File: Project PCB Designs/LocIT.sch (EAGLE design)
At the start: 5 parts, among them J1 PRT-14017

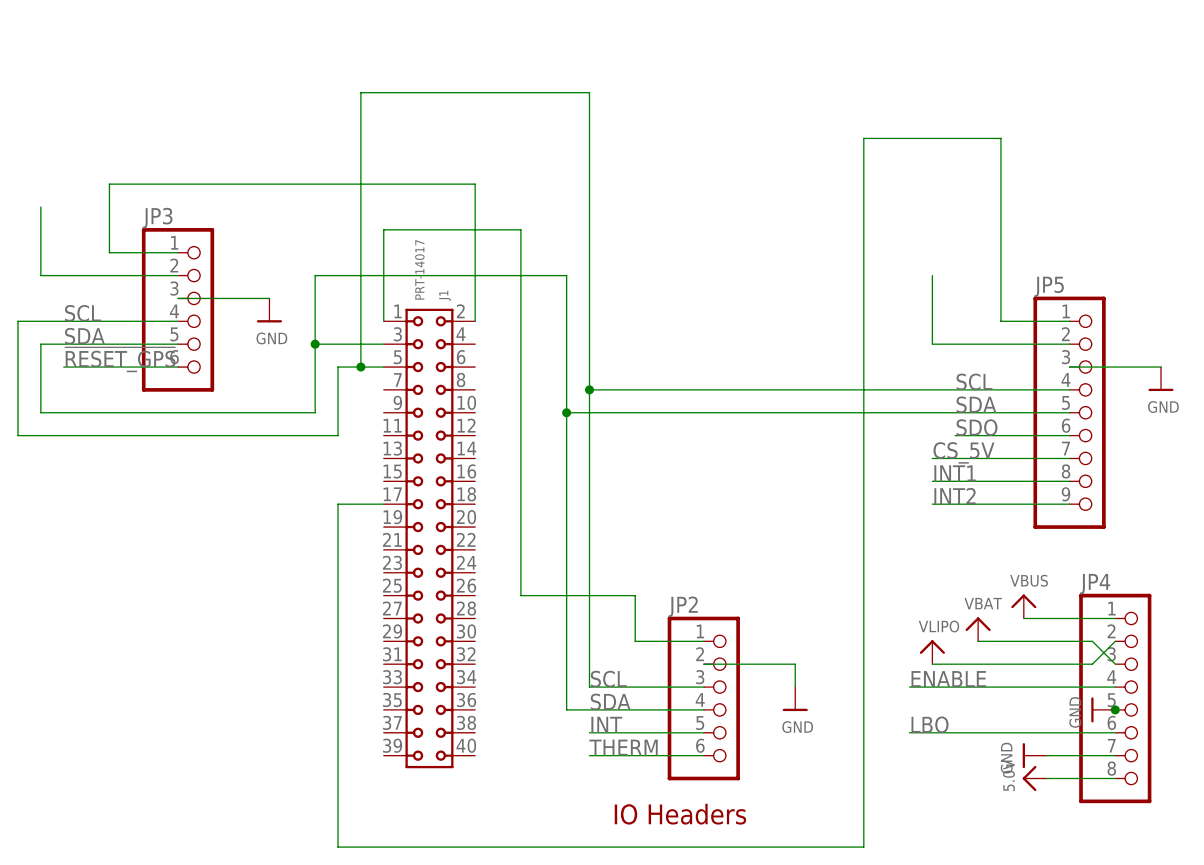
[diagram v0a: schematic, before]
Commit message: Add files via upload
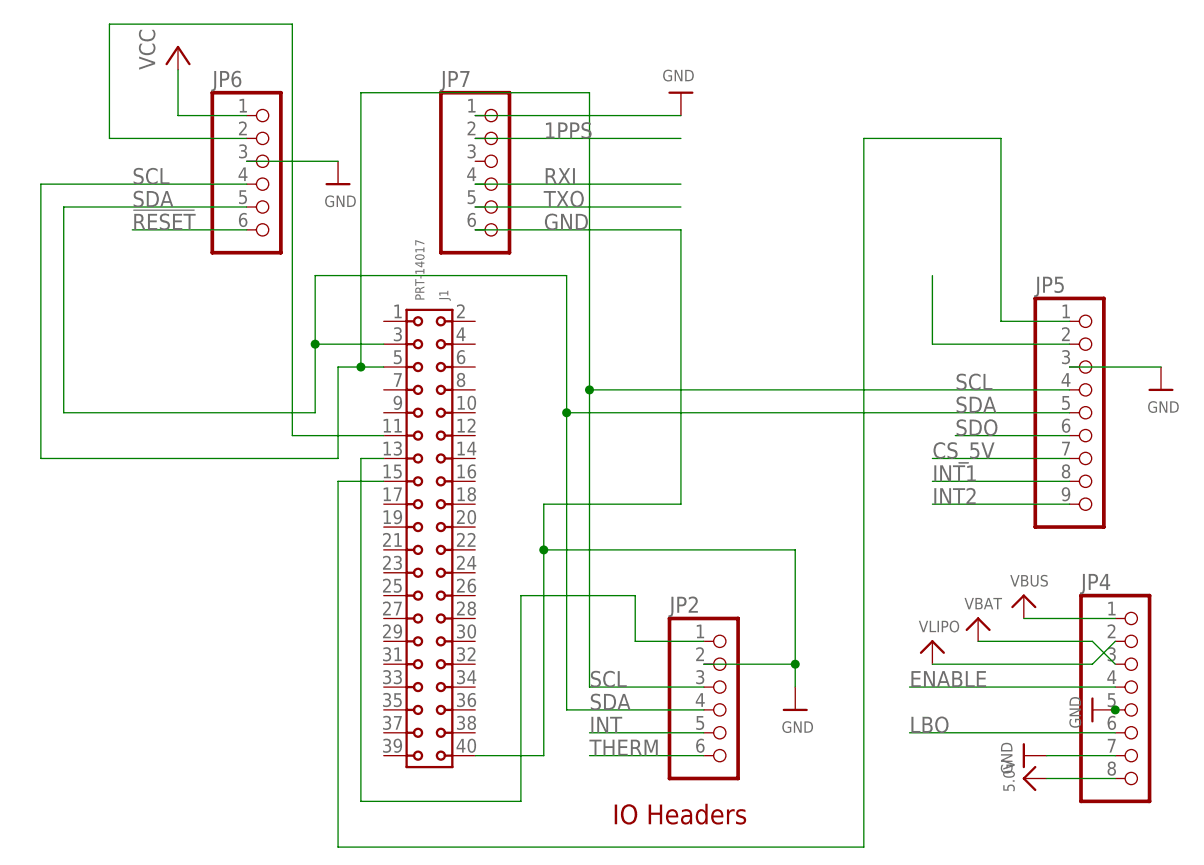
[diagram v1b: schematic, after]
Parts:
- removed JP3: (no value), microbuilder:HEADER-1X670MIL
- added JP6, JP7: (no value), microbuilder:HEADER-1X670MIL
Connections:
- removed net !RESET_GPS: JP3.6
- removed net 3.3V_GPS: JP3.2
- removed net VCC_GPS: J1.2, JP3.1
- new net !RESET: JP6.6
- new net 1PPS: JP7.2
- new net N$1: J1.11, JP6.2
- new net RXI: JP7.4
- new net TXO: JP7.5
- new net VCC: JP6.1
- net GND: now also J1.40, JP6.3, JP7.1, JP7.6; no longer JP3.3
- net SCL: now also JP6.4; no longer JP3.4
- net SDA: now also JP6.5; no longer JP3.5
- net VCC1: now also J1.13; no longer J1.1
- net VCC_GYRO: now also J1.15; no longer J1.17
